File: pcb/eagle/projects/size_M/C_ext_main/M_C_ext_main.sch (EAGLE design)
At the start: 18 parts

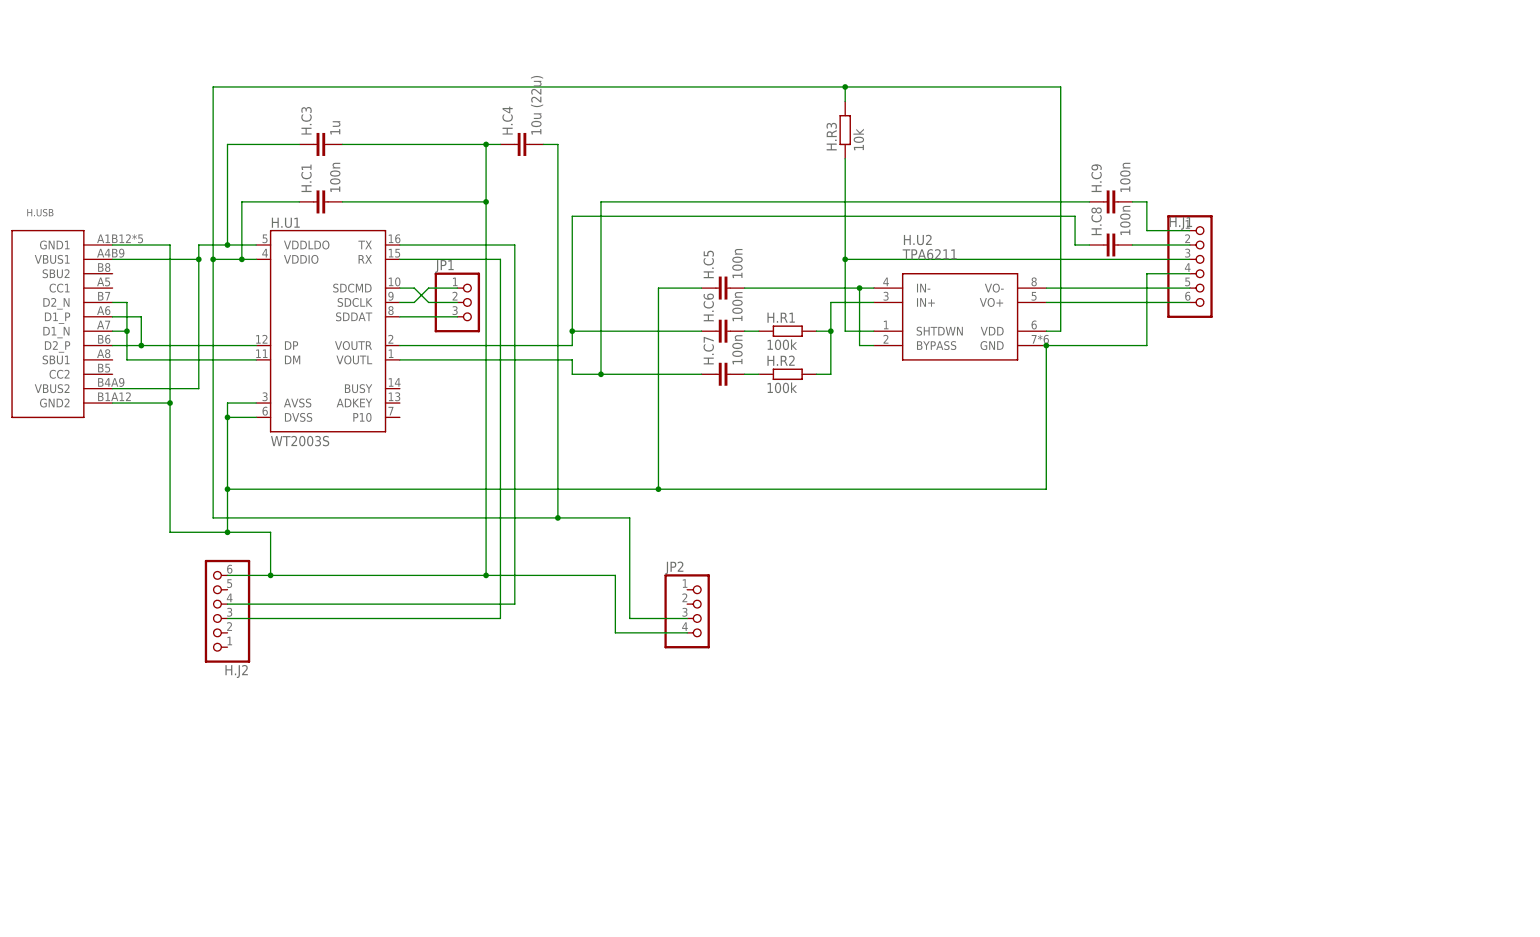
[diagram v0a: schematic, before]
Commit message: PCB M.1
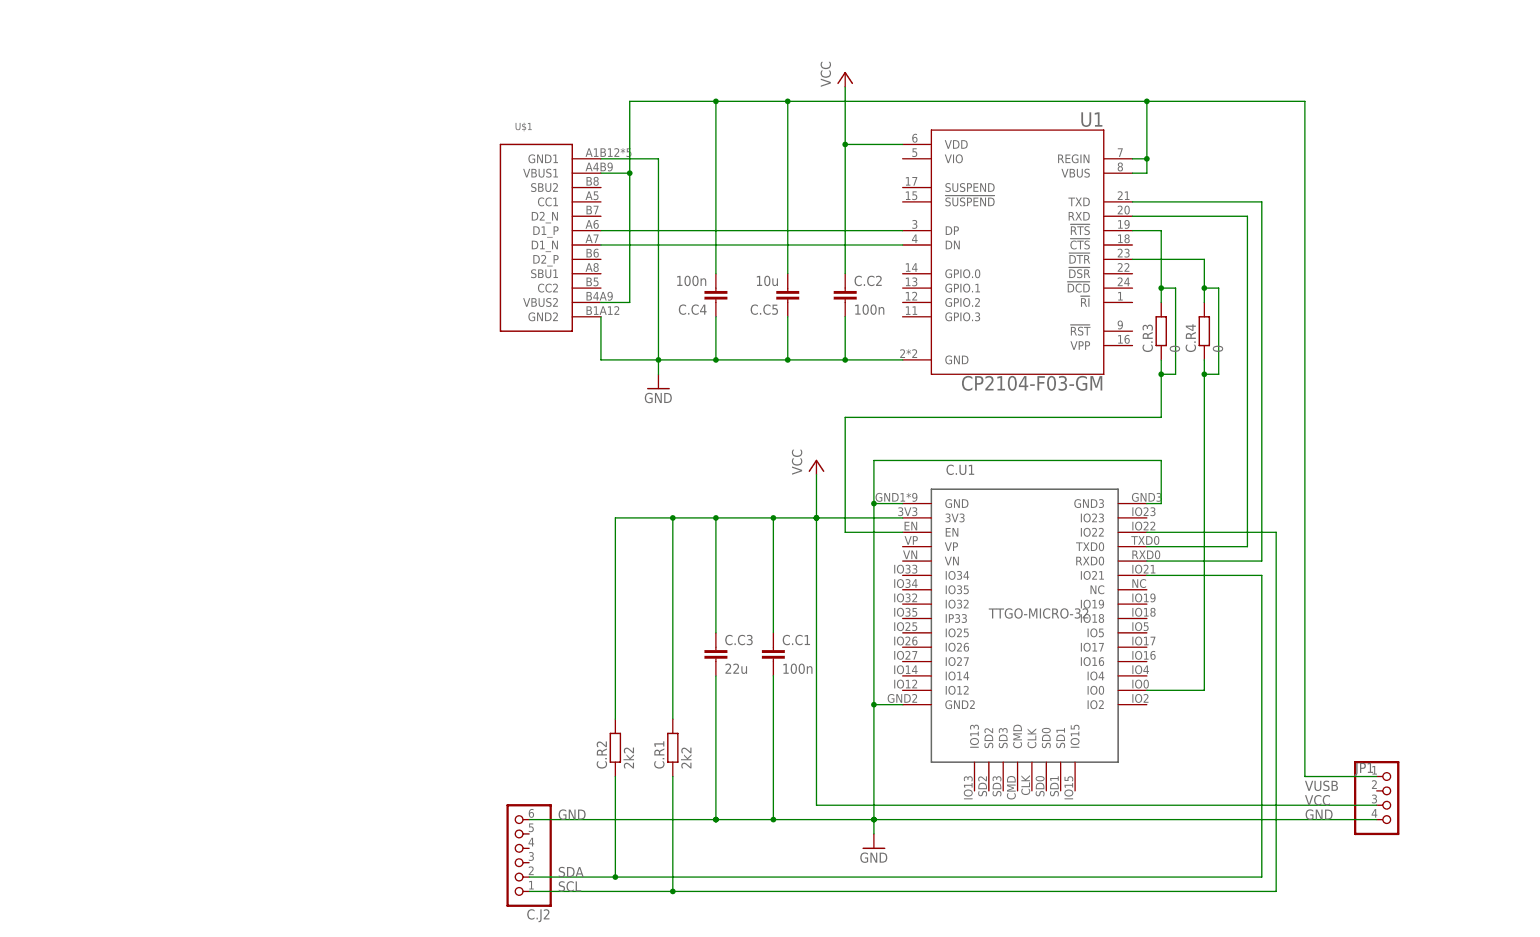
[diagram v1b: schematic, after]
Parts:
- removed H.C1, H.C5, H.C6, H.C7, H.C8, H.C9: 100n, rcl:C-EUC0603
- removed H.C3: 1u, rcl:C-EUC0603
- removed H.C4: 10u (22u), rcl:C-EUC0805
- removed H.J1, H.J2: (no value), pinhead2:PINHD-1X6
- removed H.R1, H.R2: 100k, rcl:R-EU_R0603
- removed H.R3: 10k, rcl:R-EU_R0603
- removed H.U1: WT2003S, WT2003S:WT2003S
- removed H.U2: TPA6211, hugo:TPA6211
- removed H.USB: USB-C, hugo:USB-C
- removed JP2: (no value), pinhead2:PINHD-1X4
- added C.C1, C.C2, C.C4: 100n, rcl:C-EUC0603
- added C.C3: 22u, rcl:C-EUC0805
- added C.C5: 10u, rcl:C-EUC0603
- added C.J2: (no value), pinhead2:PINHD-1X6
- added C.R1, C.R2: 2k2, rcl:R-EU_R0603
- added C.R3, C.R4: 0, rcl:R-EU_R0603
- added C.U1: TTGO-MICRO-32, hugo:TTGO-MICRO-32
- added U$1: USB-C, hugo:USB-C
- added U1: CP2104-F03-GM, CP2104:CP2104-F03-GM
- JP1: device pinhead2:PINHD-1X3 -> pinhead2:PINHD-1X4
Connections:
- removed net N$10: H.U1.DM, H.USB.D1_N, H.USB.D2_N
- removed net N$11: H.C3.1, H.U1.VDDLDO, H.USB.VBUS1, H.USB.VBUS2
- removed net N$12: H.C6.1, H.C8.1, H.U1.VOUTR
- removed net N$13: H.C7.1, H.C9.1, H.U1.VOUTL
- removed net N$14: H.R1.2, H.R2.2, H.U2.IN+
- removed net N$15: H.C5.2, H.U2.BYPASS, H.U2.IN-
- removed net N$16: H.U1.SDCLK, JP1.1
- removed net N$17: H.C6.2, H.R1.1
- removed net N$18: H.C7.2, H.R2.1
- removed net N$19: H.U1.SDDAT, JP1.3
- removed net N$3: H.J1.5, H.U2.VO-
- removed net N$4: H.J2.3, H.U1.RX
- removed net N$5: H.J2.4, H.U1.TX
- removed net N$6: H.J1.6, H.U2.VO+
- removed net N$7: H.J1.3, H.R3.1, H.U2.SHTDWN
- removed net N$8: H.U1.SDCMD, JP1.2
- removed net N$9: H.U1.DP, H.USB.D1_P, H.USB.D2_P
- new net PROG: C.R4.1, C.R4.2, C.U1.IO0, U1.!DTR
- new net RESET: C.R3.1, C.R3.2, C.U1.EN, U1.!RTS
- new net RX: C.U1.TXD0, U1.RXD
- new net SCL: C.J2.1, C.R1.1, C.U1.IO22
- new net SDA: C.J2.2, C.R2.1, C.U1.IO21
- new net TX: C.U1.RXD0, U1.TXD
- new net VUSB: C.C4.2, C.C5.2, JP1.1, U$1.VBUS1, U$1.VBUS2, U1.REGIN, U1.VBUS
- net GND: now also C.C1.2, C.C2.2, C.C3.2, C.C4.1, C.C5.1, C.J2.6, C.U1.GND, C.U1.GND2, C.U1.GND3, JP1.4, U$1.GND1, U$1.GND2, U1.GND; no longer H.C1.2, H.C3.2, H.C4.1, H.C5.1, H.J1.4, H.J2.6, H.U1.AVSS, H.U1.DVSS, H.U2.GND, H.USB.GND1, H.USB.GND2, JP2.4
- net N$1: now also U$1.D1_N, U1.DN; no longer H.C8.2, H.J1.2
- net N$2: now also U$1.D1_P, U1.DP; no longer H.C9.2, H.J1.1
- net VCC: now also C.C1.1, C.C2.1, C.C3.1, C.R1.2, C.R2.2, C.U1.3V3, JP1.3, U1.VDD; no longer H.C1.1, H.C4.2, H.R3.2, H.U1.VDDIO, H.U2.VDD, JP2.3

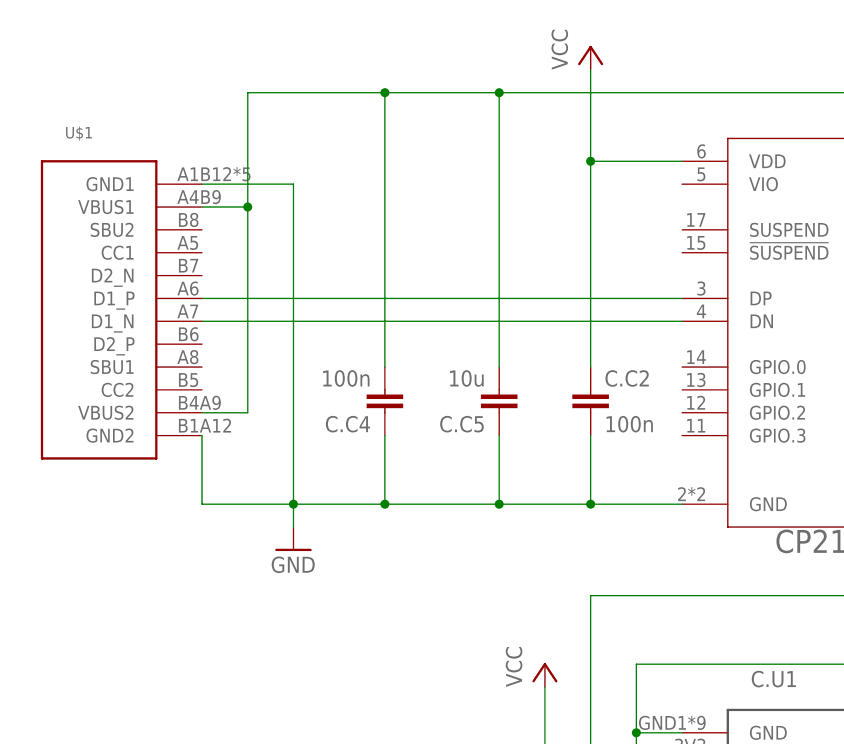
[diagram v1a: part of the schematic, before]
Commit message: updated PCBS after the version 1 delivery
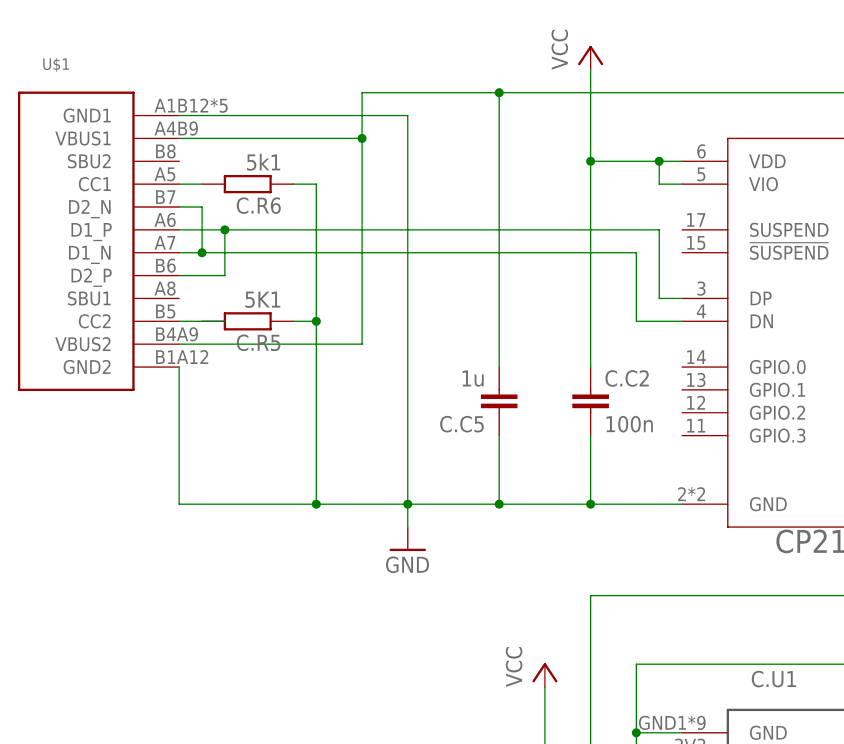
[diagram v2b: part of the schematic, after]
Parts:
- removed C.C4: 100n, rcl:C-EUC0603
- added C.R5: 5K1, rcl:R-EU_R0603
- added C.R6: 5k1, rcl:R-EU_R0603
- C.C5: value 10u -> 1u
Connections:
- new net N$3: C.R6.2, U$1.CC1
- new net N$4: C.R5.2, U$1.CC2
- net GND: now also C.R5.1, C.R6.1; no longer C.C4.1
- net N$1: now also U$1.D2_N
- net N$2: now also U$1.D2_P
- net VCC: now also U1.VIO
- net VUSB: no longer C.C4.2
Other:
- moved on the sheet: U$1

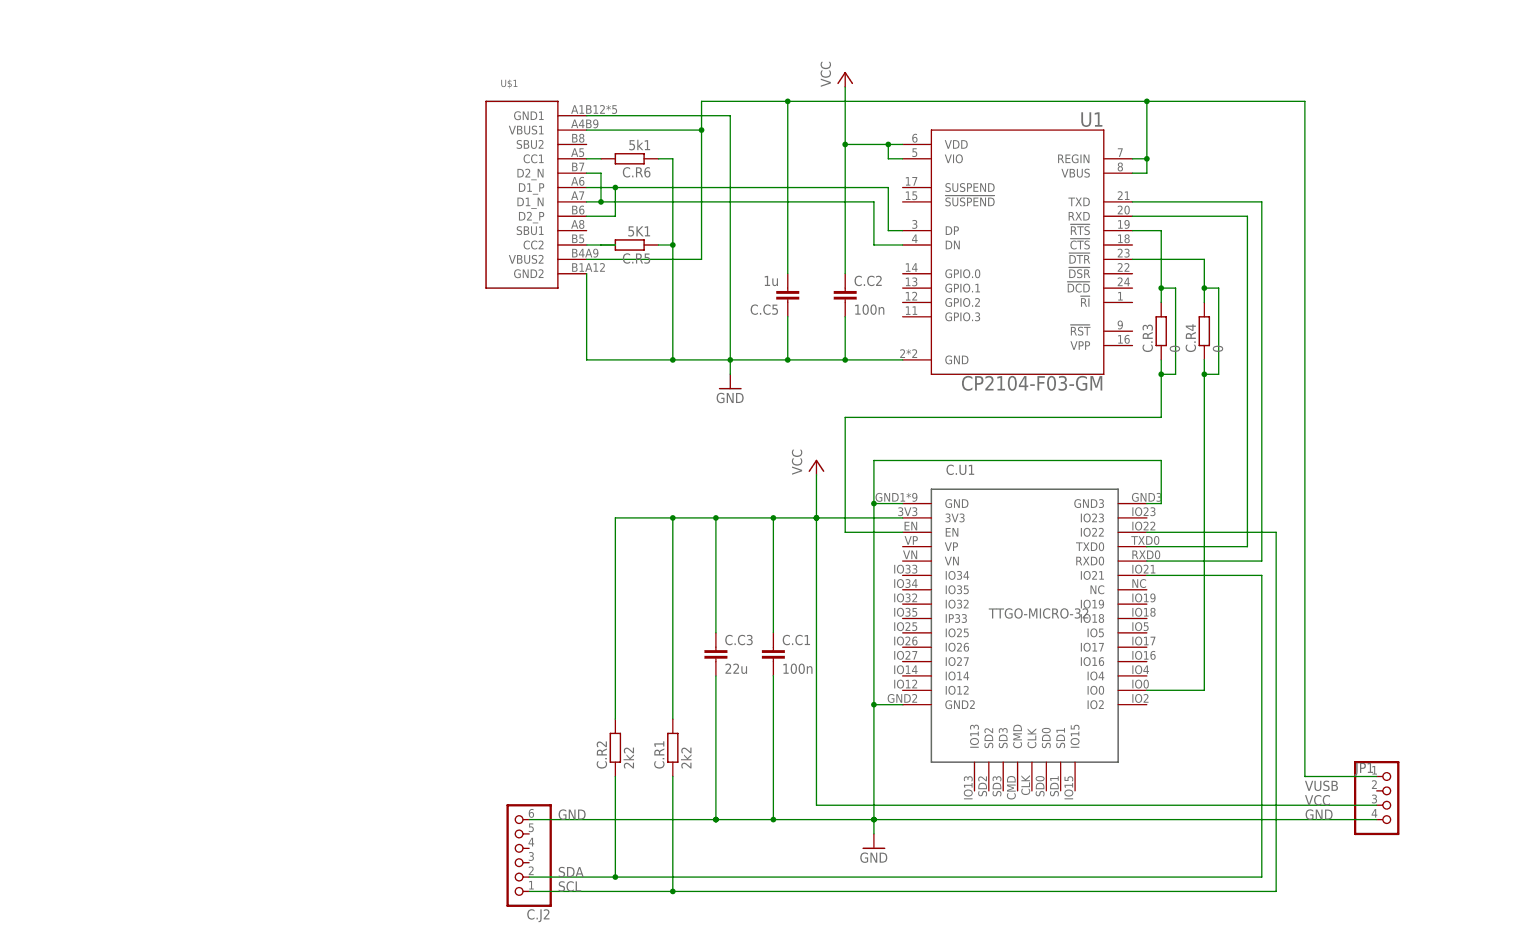
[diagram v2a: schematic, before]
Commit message: updated PCBs for version 2
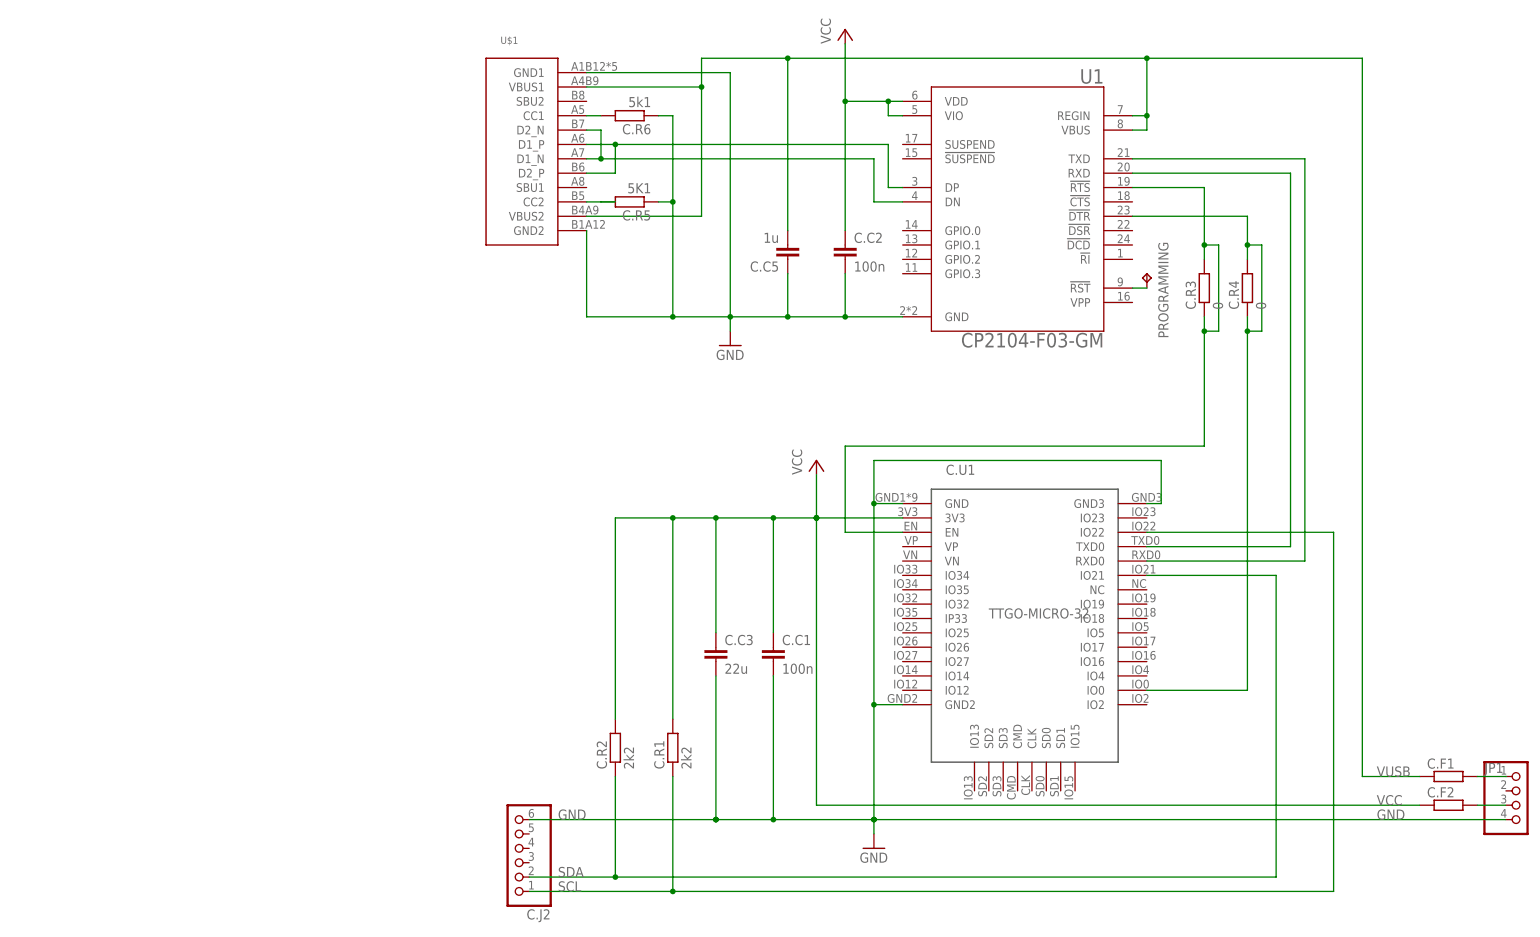
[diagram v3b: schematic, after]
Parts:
- added C.F1, C.F2: (no value), rcl:R-EU_R0805
- added PROGRAMMING: TPB1,27, testpad:TPB1,27
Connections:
- new net N$5: C.F2.2, JP1.3
- new net N$6: C.F1.2, JP1.1
- new net N$7: PROGRAMMING.TP, U1.!RST!
- net VCC: now also C.F2.1; no longer JP1.3
- net VUSB: now also C.F1.1; no longer JP1.1
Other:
- moved on the sheet: C.C2, C.C5, C.R3, C.R4, C.R5, C.R6, JP1, U$1, U1
